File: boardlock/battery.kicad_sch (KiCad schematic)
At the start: 19 parts, among them J2 Conn_01x02_MountingPin, U4 BQ27441DRZR-G1A, U5 BQ24075RGT

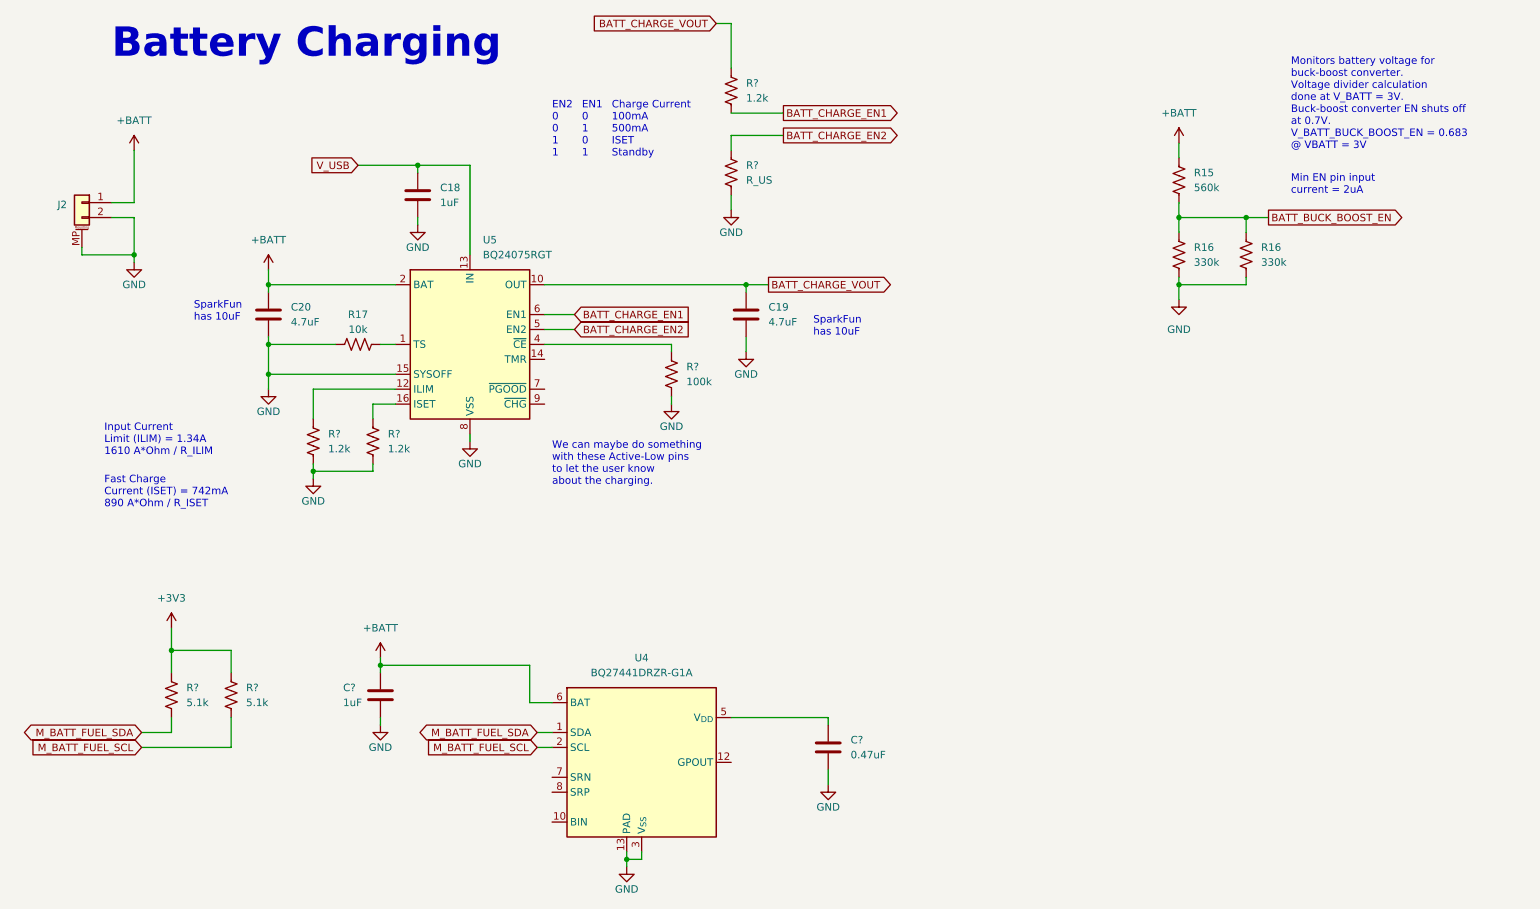
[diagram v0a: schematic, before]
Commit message: Zecong edits
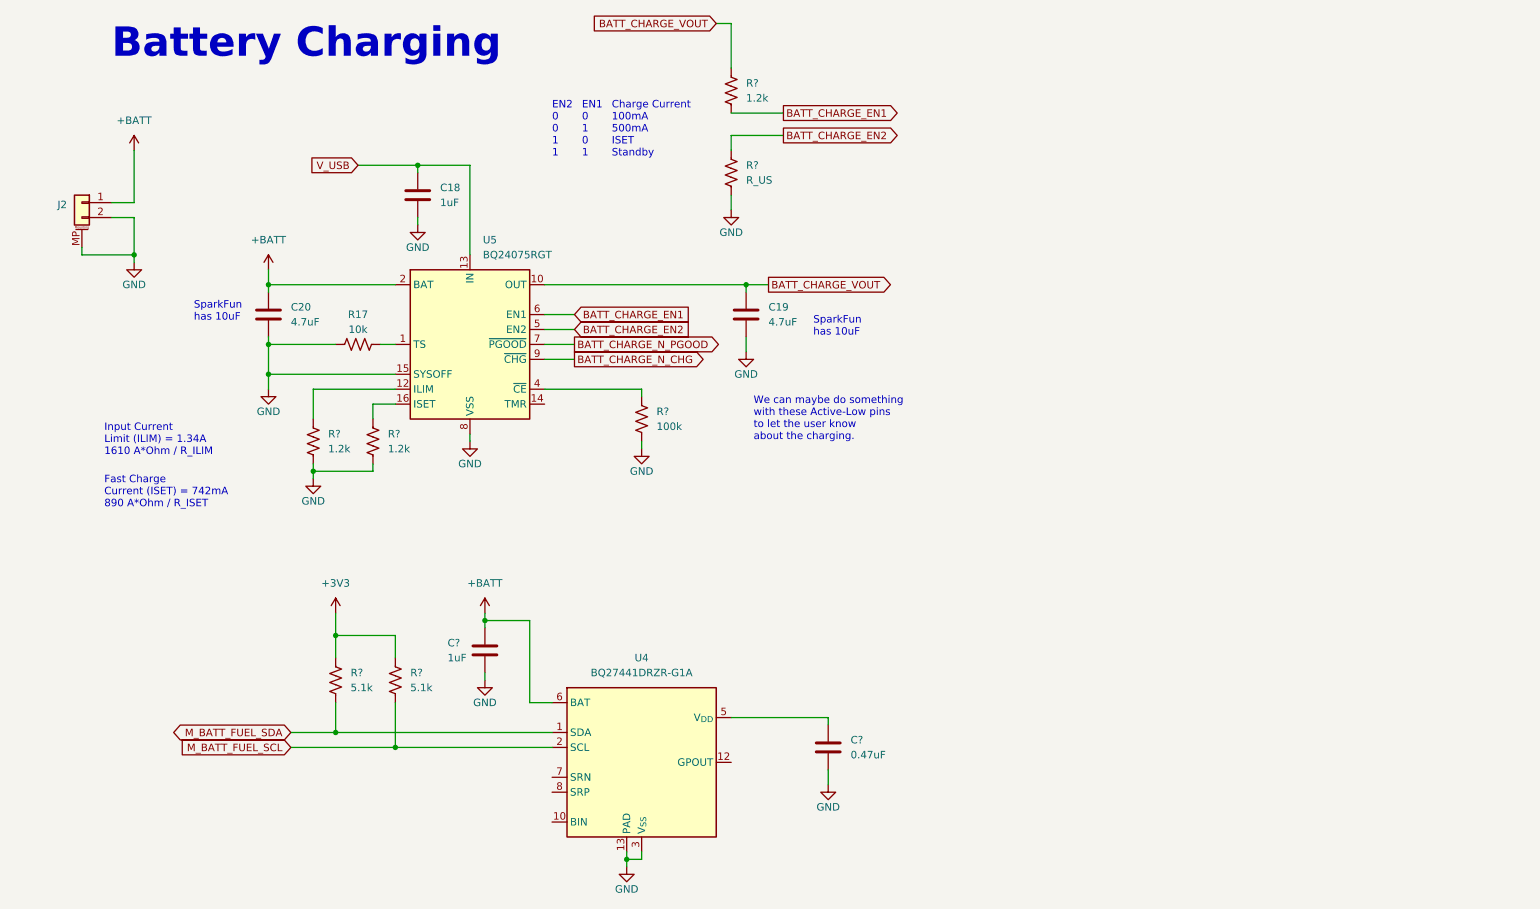
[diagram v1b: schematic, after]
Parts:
- removed R15: 560k, symbol Device:R_US
- removed R16 (x2): 330k, symbol Device:R_US
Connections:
- net BATT_CHARGE_N_PGOOD: now reaches U5.7 (~{PGOOD})
- net BATT_CHARGE_N_CHG: now reaches U5.9 (~{CHG})
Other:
- note removed: "Min EN pin input current = 2uA"
- note removed: "Monitors battery voltage for buck-boost converter. Voltage divider calculation done at V_BATT = 3V. Buck-boost converter EN shuts off at 0.7V. V_BATT_BUCK_BOOST_EN = 0.683 @ VBATT = 3V"
- moved on the sheet: C?, R?
